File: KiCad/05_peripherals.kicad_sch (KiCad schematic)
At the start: 33 parts, among them IC501 DS3231MZ+TRL, U501 BME280, U502 DS18B20, U503 LM35-LP

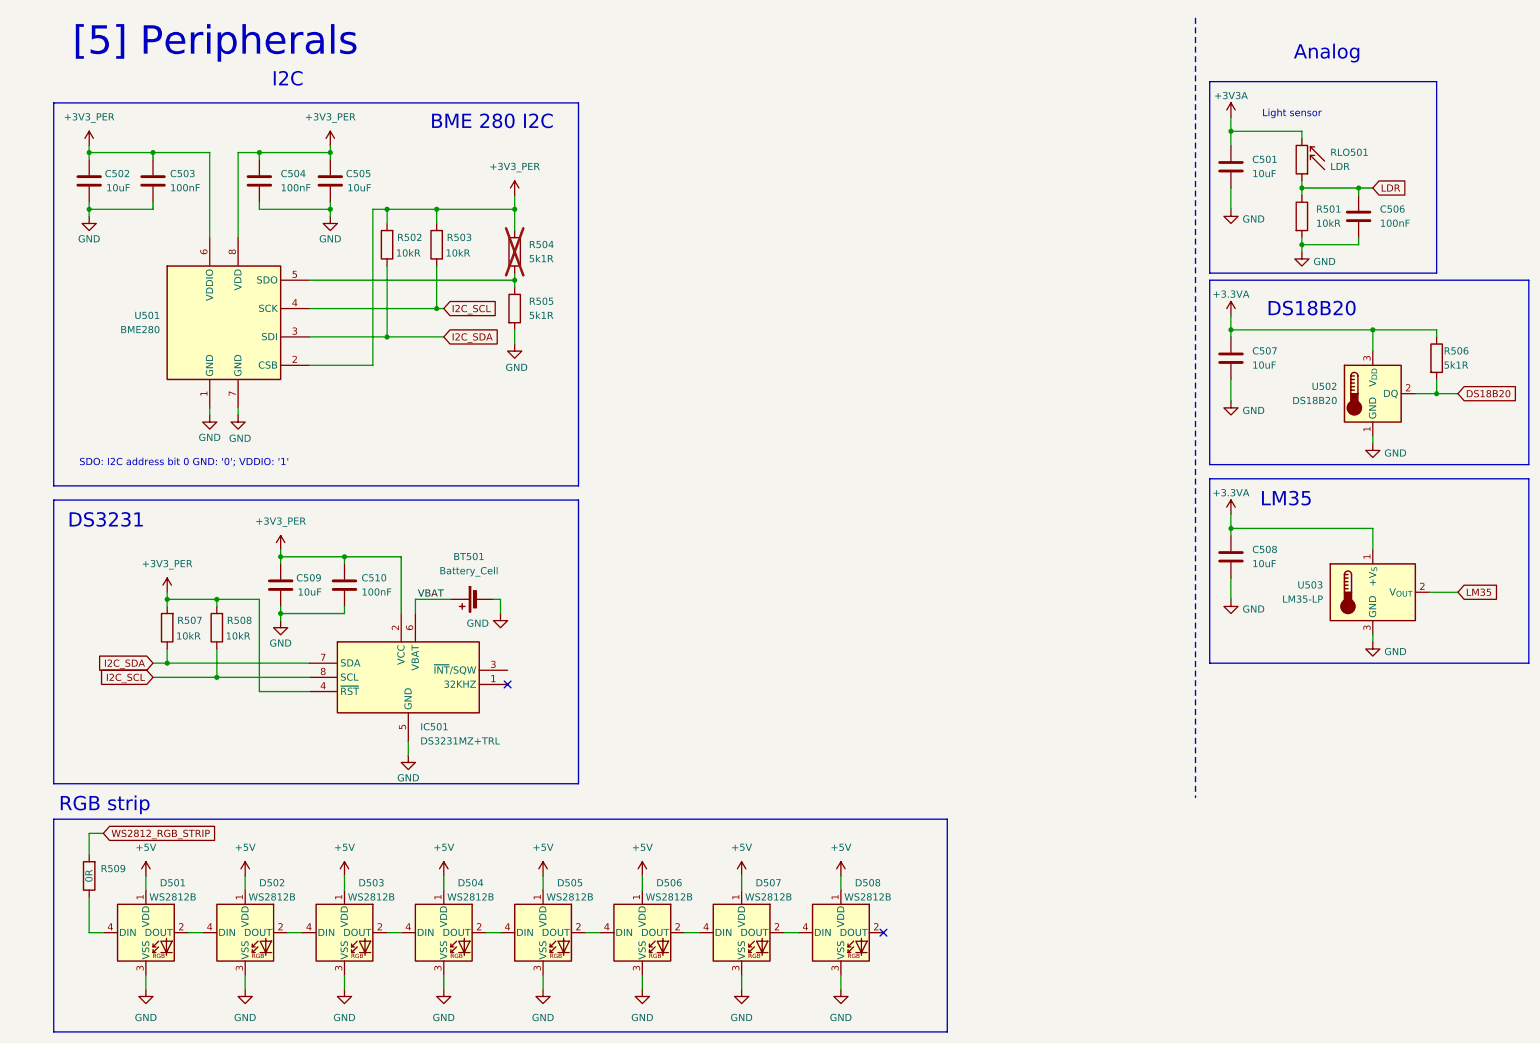
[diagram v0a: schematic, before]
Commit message: First scheme version
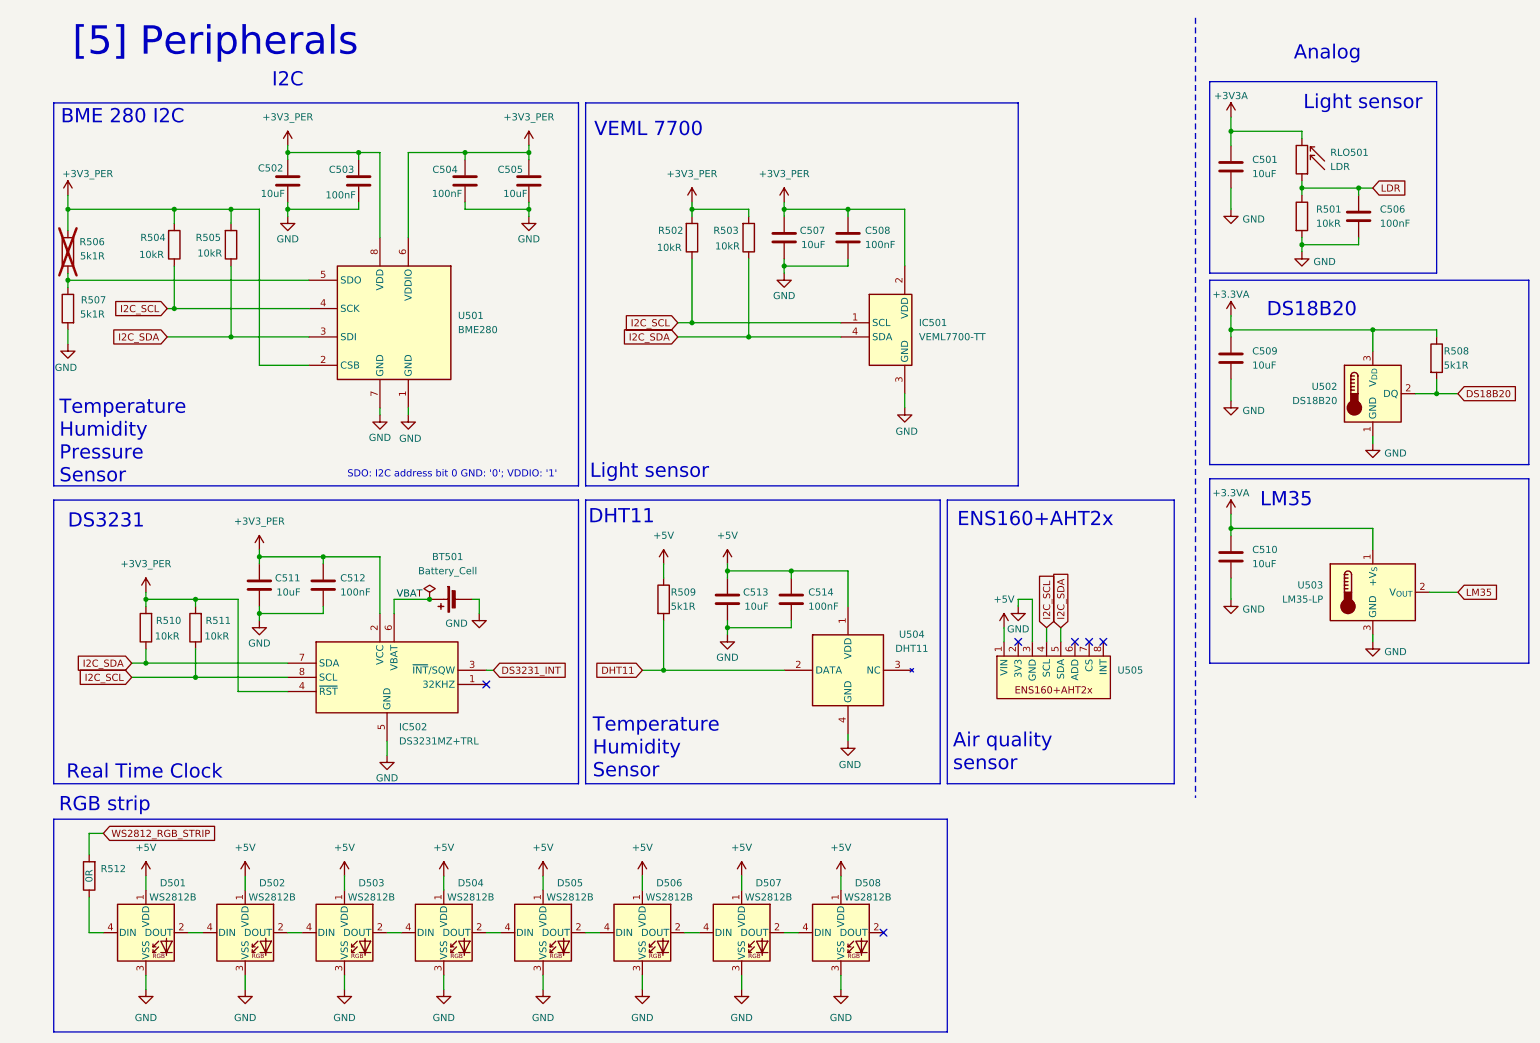
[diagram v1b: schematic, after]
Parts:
- added C507, C513: 10uF, Capacitor_SMD:C_0603_1608Metric, symbol Device:C
- added C508, C514: 100nF, Capacitor_SMD:C_0603_1608Metric, symbol Device:C
- added IC501: VEML7700-TT, esp32_s3_weather_webserver:VEML7700, symbol esp32_s3_weather_webserver:VEML7700-TT
- added R502, R503: 10kR, Resistor_SMD:R_0805_2012Metric, symbol Device:R
- added R509: 5k1R, Resistor_SMD:R_0402_1005Metric, symbol Device:R
- added U504: DHT11, esp32_s3_weather_webserver:DHT11, symbol esp32_s3_weather_webserver:DHT11
- added U505: ~, symbol esp32_s3_weather_webserver:ENS160+AHT2x
- renumbered C505 to C502, C504 to C503, C503 to C504, C502 to C505, C507 to C509, C508 to C510, C509 to C511, C510 to C512, IC501 to IC502, R503 to R504, R502 to R505, R504 to R506, R505 to R507, R506 to R508, R507 to R510, R508 to R511, R509 to R512
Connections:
- net +3V3_PER: now also C507.1, C508.1, IC501.2 (VDD), R502.2, R503.2
- net +5V: now also C513.1, C514.1, R509.1, U504.1 (VDD), U505.1 (VIN)
- net GND: now also C507.2, C508.2, C513.2, C514.2, IC501.3 (GND), U504.4 (GND), U505.3 (GND)
- net I2C_SCL: now also IC501.1 (SCL), R502.1, U505.4 (SCL)
- net I2C_SDA: now also IC501.4 (SDA), R503.1, U505.5 (SDA)
- net DS3231_INT: now reaches IC502.3 (~{INT}/SQW)
- new net DHT11: R509.2, U504.2 (DATA)
- no-connect marks 2 -> 6
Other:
- note added: "Air quality sensor"
- note added: "DHT11"
- note added: "ENS160+AHT2x"
- note added: "Real Time Clock"
- note added: "Temperature Humidity Pressure Sensor"
- note added: "Temperature Humidity Sensor"
- note added: "VEML 7700"
- moved on the sheet: BT501, C502, C503, C504, C505, C511, C512, IC502, R504, R505, R506, R507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
